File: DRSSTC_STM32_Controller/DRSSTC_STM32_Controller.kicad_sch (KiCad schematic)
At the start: 21 parts, among them J1 Conn_01x04, J10 Conn_01x04, J11 Conn_01x04, J12 Conn_01x10, J13 USB_C_Receptacle_USB2.0_14P, J14 Conn_01x10, J16 Conn_01x04, J17 Conn_01x10, J32 Screw_Terminal_01x02, J33 Screw_Terminal_01x02, J4 Screw_Terminal_01x02, J42 Screw_Terminal_01x02, J5 Conn_Coaxial, J6 Conn_Coaxial, J7 Conn_01x04

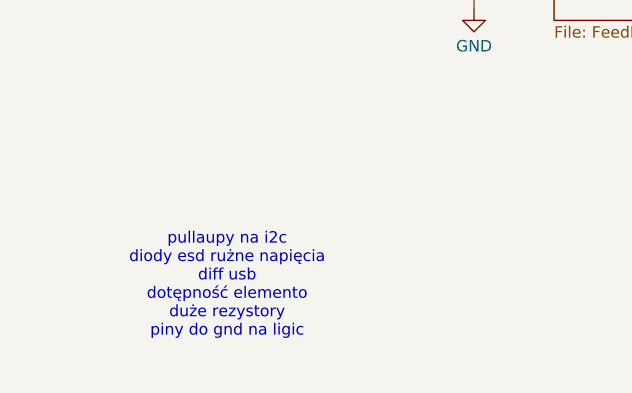
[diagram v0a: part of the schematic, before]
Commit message: finalize the controller design
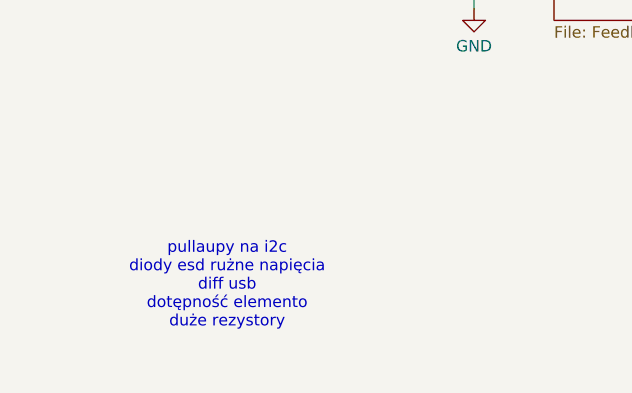
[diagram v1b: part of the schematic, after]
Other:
- note added: "pullaupy na i2c diody esd rużne napięcia diff usb dotępność elemento duże rezystory"
- note removed: "pullaupy na i2c diody esd rużne napięcia diff usb dotępność elemento duże rezystory piny do gnd na ligic"
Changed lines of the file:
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@@
 		)
 	)
-	(text "pullaupy na i2c\ndiody esd rużne napięcia\ndiff usb\ndotępność elemento\nduże rezystory\npiny do gnd na ligic"
+	(text "pullaupy na i2c\ndiody esd rużne napięcia\ndiff usb\ndotępność elemento\nduże rezystory\n"
 		(exclude_from_sim no)
 		(at 41.148 255.524 0)
